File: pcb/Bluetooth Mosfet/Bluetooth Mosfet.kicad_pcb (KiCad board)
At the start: 2 copper layers, 43.2 x 30.5 mm, 10 parts, among them J1 1x3 Header, J2 1x4 Header, J3 1x2 Header, Q1 IRF510N, U2 ATtiny 1614

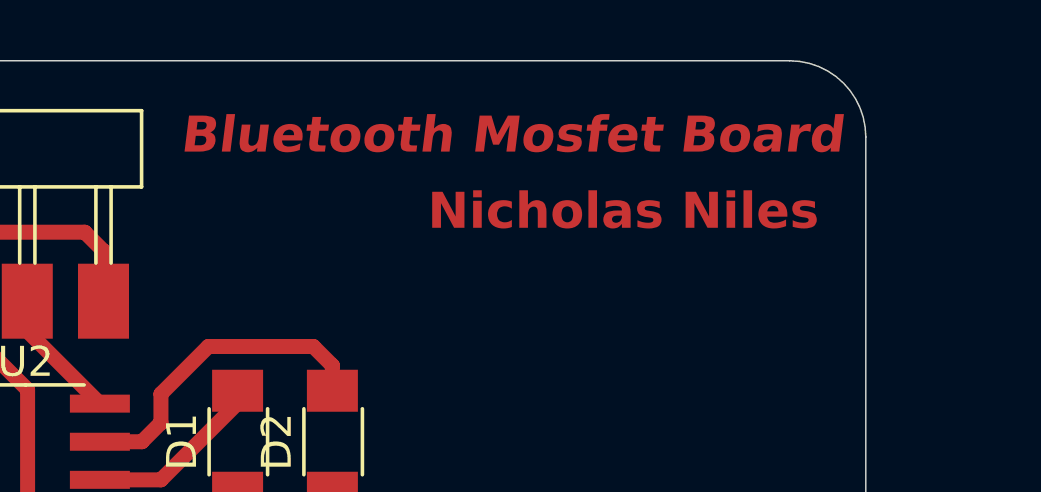
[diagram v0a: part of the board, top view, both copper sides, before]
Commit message: Text update
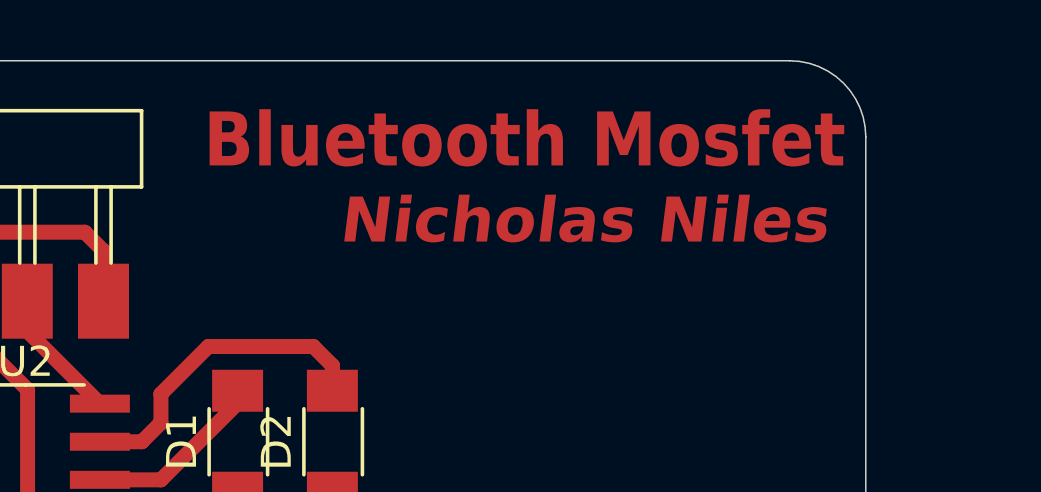
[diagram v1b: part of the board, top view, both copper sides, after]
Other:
- board text added: "Bluetooth Mosfet"
- board text removed: "Bluetooth Mosfet Board"
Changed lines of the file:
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@@
 				(font
 					(size 1.27 1.27)
+					(thickness 0.15)
 				)
 			)
@@
 				(font
 					(size 1.27 1.27)
+					(thickness 0.15)
 				)
 			)
@@
 				(font
 					(size 1.27 1.27)
+					(thickness 0.15)
 				)
 			)
@@
 				(font
 					(size 1.27 1.27)
+					(thickness 0.15)
 				)
 			)
@@
 				(font
 					(size 1.27 1.27)
+					(thickness 0.15)
 				)
 			)
@@
 				(font
 					(size 1.27 1.27)
+					(thickness 0.15)
 				)
 			)
@@
 				(font
 					(size 1.27 1.27)
+					(thickness 0.15)
 				)
 			)
@@
 				(font
 					(size 1.27 1.27)
+					(thickness 0.15)
 				)
 			)
@@
 				(font
 					(size 1.27 1.27)
+					(thickness 0.15)
 				)
 			)
@@
 				(font
 					(size 1.27 1.27)
+					(thickness 0.15)
 				)
 			)
@@
 				(font
 					(size 1.27 1.27)
+					(thickness 0.15)
 				)
 			)
@@
 				(font
 					(size 1.27 1.27)
+					(thickness 0.15)
 				)
 			)
@@
 				(font
 					(size 1.27 1.27)
+					(thickness 0.15)
 				)
 			)
@@
 				(font
 					(size 1.27 1.27)
+					(thickness 0.15)
 				)
 			)
@@
 				(font
 					(size 1.27 1.27)
+					(thickness 0.15)
 				)
 			)
@@
 				(font
 					(size 1.27 1.27)
+					(thickness 0.15)
 				)
 			)
@@
 				(font
 					(size 1.27 1.27)
+					(thickness 0.15)
 				)
 			)
@@
 				(font
 					(size 1.27 1.27)
+					(thickness 0.15)
 				)
 			)
@@
 				(font
 					(size 1.27 1.27)
+					(thickness 0.15)
 				)
 			)
@@
 				(font
 					(size 1.27 1.27)
+					(thickness 0.15)
 				)
 			)
@@
 				(font
 					(size 1.27 1.27)
+					(thickness 0.15)
 				)
 			)
@@
 				(font
 					(size 1.27 1.27)
+					(thickness 0.15)
 				)
 			)
@@
 				(font
 					(size 1.27 1.27)
+					(thickness 0.15)
 				)
 			)
@@
 				(font
 					(size 1.27 1.27)
+					(thickness 0.15)
 				)
 			)
@@
 				(font
 					(size 1.27 1.27)
+					(thickness 0.15)
 				)
 			)
@@
 				(font
 					(size 1.27 1.27)
+					(thickness 0.15)
 				)
 			)
@@
 				(font
 					(size 1.27 1.27)
+					(thickness 0.15)
 				)
 			)
@@
 				(font
 					(size 1.27 1.27)
+					(thickness 0.15)
 				)
 			)
@@
 				(font
 					(size 1.27 1.27)
+					(thickness 0.15)
 				)
 			)
@@
 				(font
 					(size 1.27 1.27)
+					(thickness 0.15)
 				)
 			)
@@
 		(layer "Edge.Cuts")
 	)
-	(gr_text "Bluetooth Mosfet Board"
-		(at 62.215 48.465 0)
+	(gr_text "Bluetooth Mosfet"
+		(at 63 49 0)
 		(layer "F.Cu")
 		(effects
 			(font
-				(size 1.2 1.2)
-				(thickness 0.24)
+				(size 1.8 1.6)
+				(thickness 0.35)
 				(bold yes)
-				(italic yes)
 			)
 			(justify left bottom)
@@
 	)
 	(gr_text "Nicholas Niles"
-		(at 70.47 51.005 0)
+		(at 67.5 51.5 0)
 		(layer "F.Cu")
 		(effects
 			(font
-				(size 1.2 1.2)
+				(size 1.5 1.5)
 				(thickness 0.24)
 				(bold yes)
+				(italic yes)
 			)
 			(justify left bottom)
